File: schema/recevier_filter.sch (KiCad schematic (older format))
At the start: 9 parts

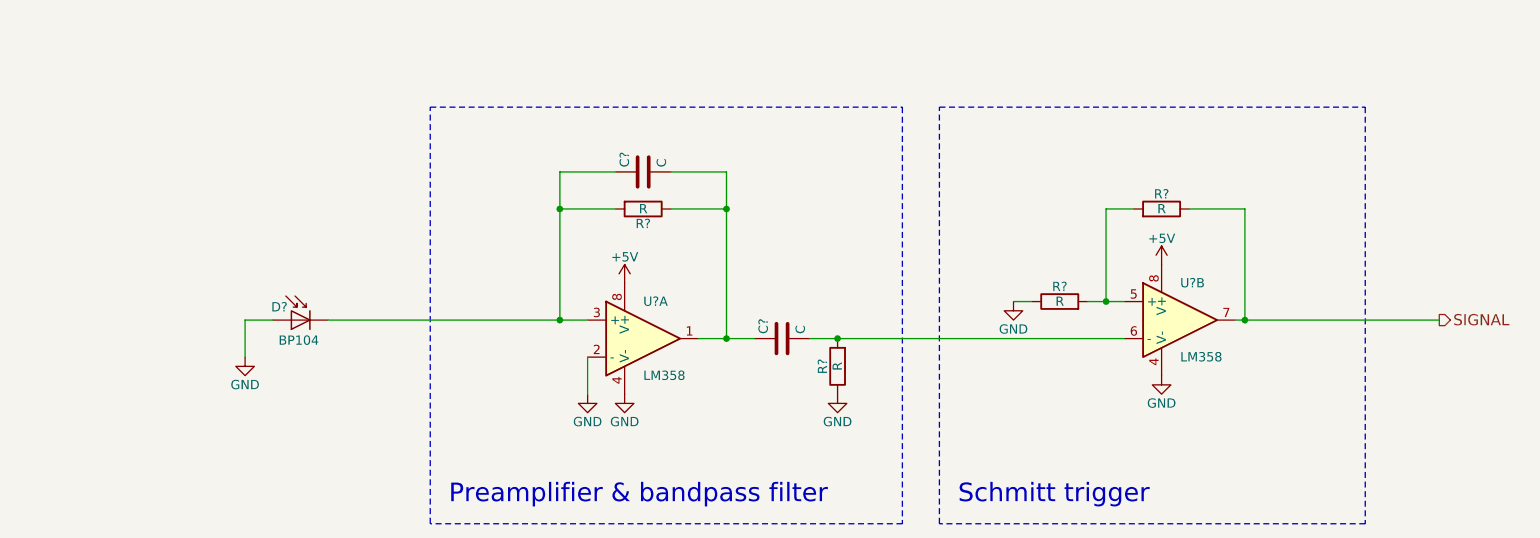
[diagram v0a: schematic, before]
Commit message: some filter modif
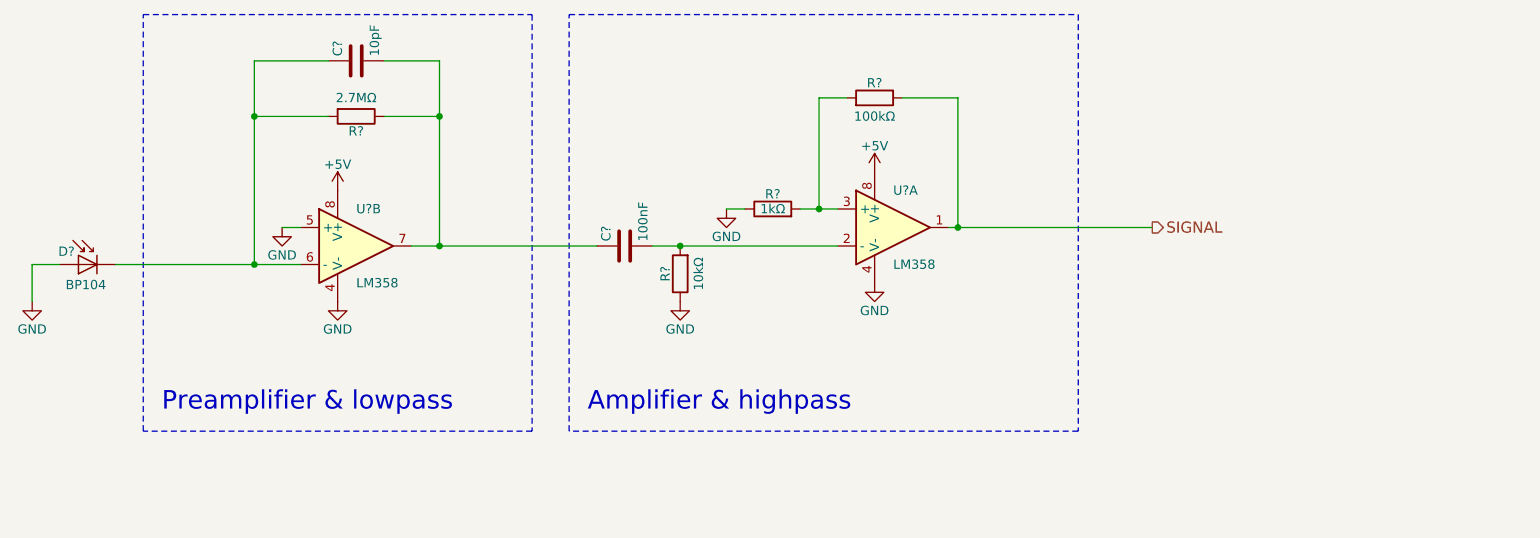
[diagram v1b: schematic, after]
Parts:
- removed C?: C, symbol C
- added C?: 10pF, symbol C
- C?: value C -> 100nF
- R?: value R -> 10kΩ
- R?: value R -> 2.7MΩ
- R?: value R -> 100kΩ
- R?: value R -> 1kΩ
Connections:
- net GND: now also U?.5 (+); no longer U?.2 (-)
- net SIGNAL: now also U?.1; no longer U?.7
- net at D?.1 (K), R?.2: now also U?.6 (-), C?.1; no longer U?.3 (+)
- net at C?.2, R?.2: now also U?.2 (-); no longer U?.6 (-)
- net at C?.1, R?.1: now also U?.7, C?.2; no longer U?.1
- net at R?.2, R?.2: now also U?.3 (+); no longer U?.5 (+)
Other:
- note added: "Amplifier & highpass"
- note added: "Preamplifier & lowpass"
- note removed: "Preamplifier & bandpass filter"
- note removed: "Schmitt trigger"
- moved on the sheet: C?, D?, R?
